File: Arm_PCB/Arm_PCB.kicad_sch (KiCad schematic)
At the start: 28 parts, among them J1 Conn_02x04_Counter_Clockwise, J10 Conn_02x02_Counter_Clockwise, J11 Conn_02x04_Counter_Clockwise, J12 Screw_Terminal_01x02, J13 Screw_Terminal_01x02, J14 Screw_Terminal_01x02, J15 Screw_Terminal_01x02, J16 Screw_Terminal_01x02, J17 Screw_Terminal_01x02, J18 Screw_Terminal_01x02, J2 Conn_02x04_Counter_Clockwise, J3 Conn_02x04_Counter_Clockwise, J4 Conn_02x04_Counter_Clockwise, J5 Conn_02x03_Counter_Clockwise, J7 Conn_02x03_Counter_Clockwise, J8 Conn_02x02_Counter_Clockwise, J9 Conn_02x04_Counter_Clockwise, SW1 SW_Push, SW2 SW_Push, SW3 SW_Push, SW4 SW_Push

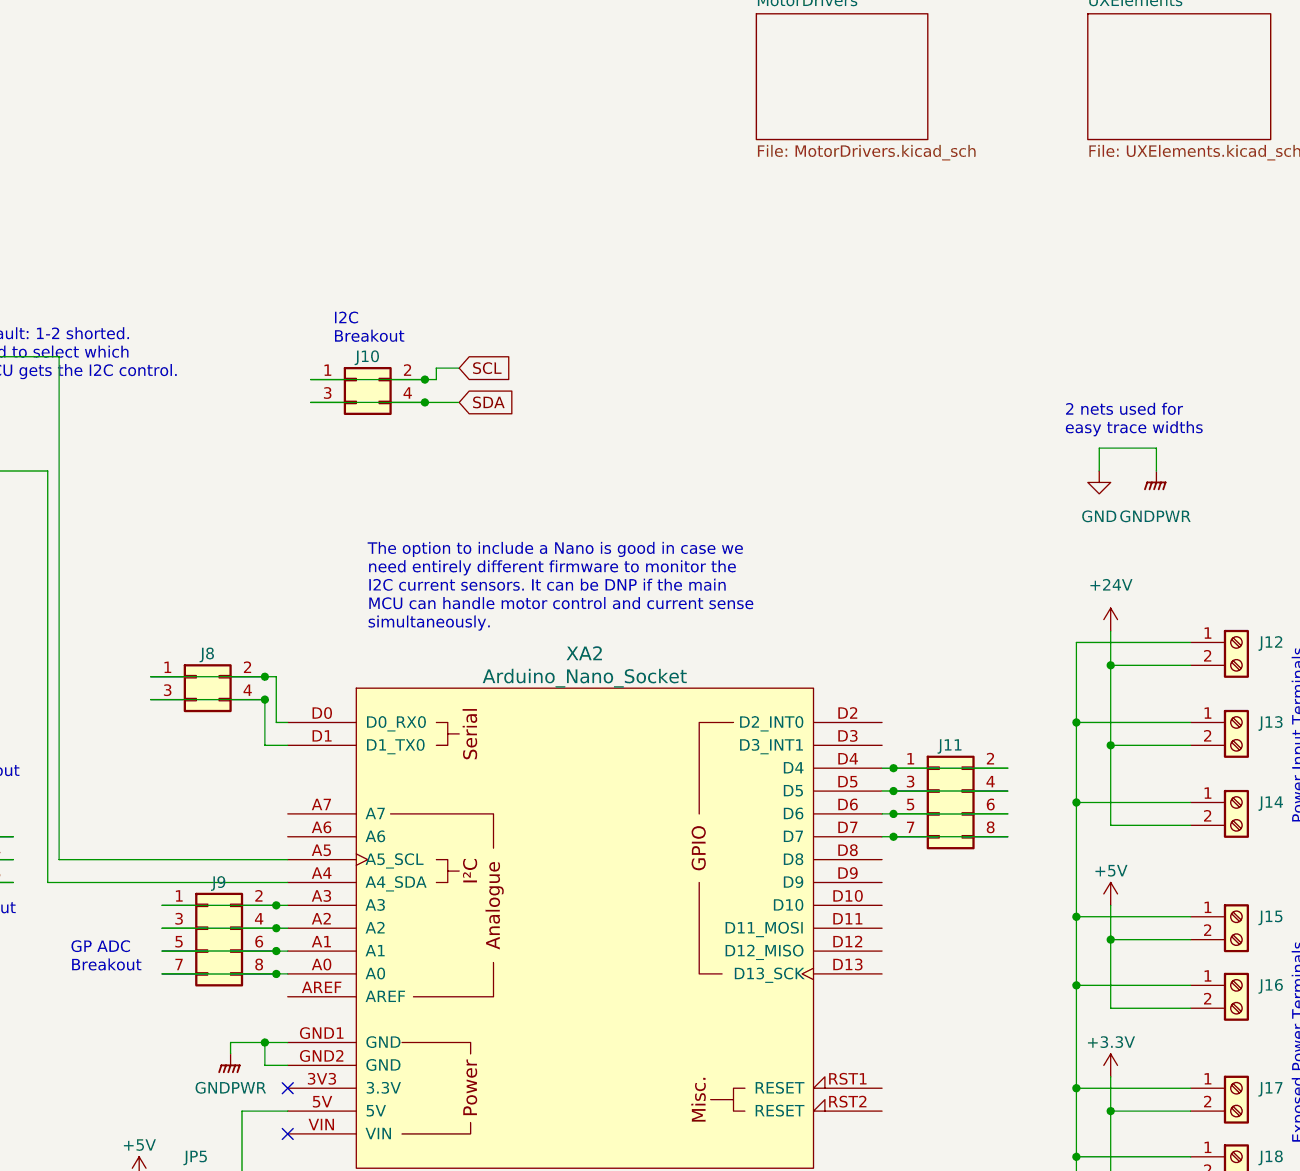
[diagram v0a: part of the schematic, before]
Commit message: Continue layout, pick some components
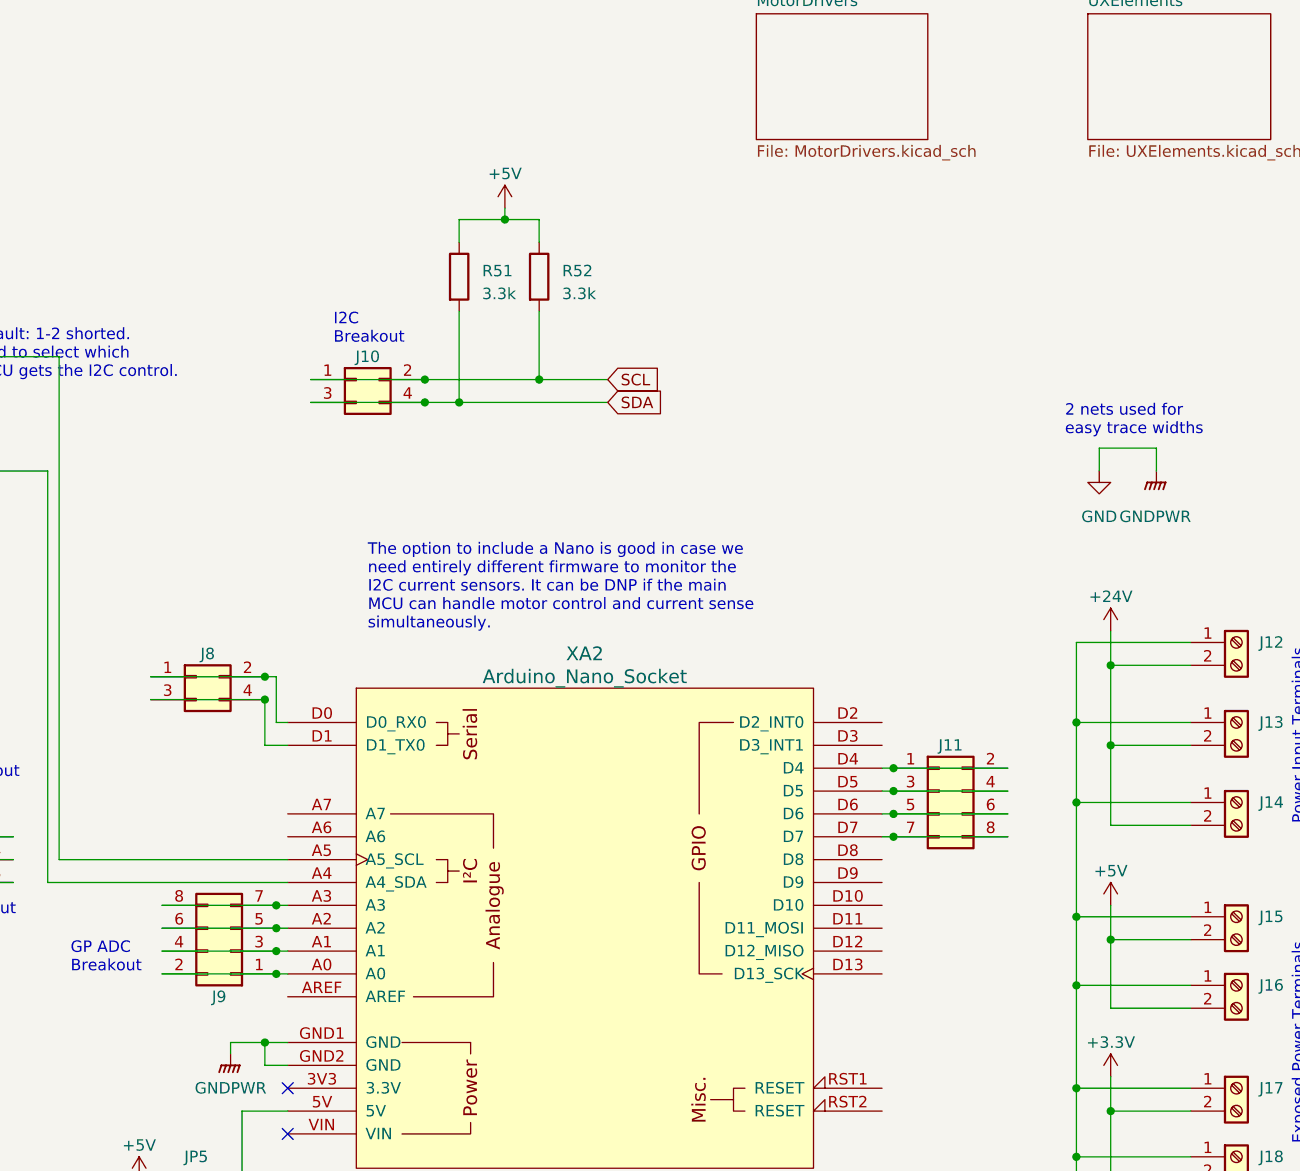
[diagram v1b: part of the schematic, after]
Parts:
- added R51, R52: 3.3k, Resistor_SMD:R_1206_3216Metric_Pad1.30x1.75mm_HandSolder, symbol Device:R
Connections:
- net +5V: now also R51.1, R52.1
- net SCL: now also R52.2
- net SDA: now also R51.2
- net at J9.7 (Pin_7), J9.8 (Pin_8): now also XA2.A3; no longer XA2.A0
- net at J9.5 (Pin_5), J9.6 (Pin_6): now also XA2.A2; no longer XA2.A1
- net at J9.3 (Pin_3), J9.4 (Pin_4): now also XA2.A1; no longer XA2.A2
- net at J9.1 (Pin_1), J9.2 (Pin_2): now also XA2.A0; no longer XA2.A3
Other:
- moved on the sheet: J9
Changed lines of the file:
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@@
   (junction (at 95.25 110.49) (diameter 0) (color 0 0 0 0)
   )
+  (junction (at 176.53 62.23) (diameter 0) (color 0 0 0 0)
+  )
   (junction (at 105.41 118.11) (diameter 0) (color 0 0 0 0)
   )
@@
   (junction (at 24.13 173.99) (diameter 0) (color 0 0 0 0)
   )
+  (junction (at 172.72 44.45) (diameter 0) (color 0 0 0 0)
+  )
   (junction (at 24.13 176.53) (diameter 0) (color 0 0 0 0)
   )
@@
   )
   (junction (at 215.9 113.03) (diameter 0) (color 0 0 0 0)
+  )
+  (junction (at 167.64 64.77) (diameter 0) (color 0 0 0 0)
   )
   (junction (at 26.67 118.11) (diameter 0) (color 0 0 0 0)
@@
   (no_connect (at 148.59 140.97))
   (no_connect (at 27.94 191.77))
+  (wire (pts (xy 176.53 46.99) (xy 176.53 44.45))
+    (stroke (width 0) (type default))
+  )
   (wire (pts (xy 93.98 120.65) (xy 96.52 120.65))
     (stroke (width 0) (type default))
@@
     (stroke (width 0) (type default))
   )
+  (wire (pts (xy 167.64 44.45) (xy 167.64 46.99))
+    (stroke (width 0) (type default))
+  )
   (wire (pts (xy 146.05 97.79) (xy 133.35 97.79))
     (stroke (width 0) (type default))
@@
     (stroke (width 0) (type default))
   )
+  (wire (pts (xy 176.53 54.61) (xy 176.53 62.23))
+    (stroke (width 0) (type default))
+  )
   (wire (pts (xy 95.25 107.95) (xy 107.95 107.95))
     (stroke (width 0) (type default))
@@
     (stroke (width 0) (type default))
   )
+  (wire (pts (xy 172.72 43.18) (xy 172.72 44.45))
+    (stroke (width 0) (type default))
+  )
   (wire (pts (xy 240.03 120.65) (xy 240.03 124.46))
     (stroke (width 0) (type default))
   )
+  (wire (pts (xy 167.64 64.77) (xy 184.15 64.77))
+    (stroke (width 0) (type default))
+  )
   (wire (pts (xy 96.52 125.73) (xy 93.98 125.73))
     (stroke (width 0) (type default))
@@
     (stroke (width 0) (type default))
   )
+  (wire (pts (xy 167.64 54.61) (xy 167.64 64.77))
+    (stroke (width 0) (type default))
+  )
   (wire (pts (xy 240.03 93.98) (xy 248.92 93.98))
     (stroke (width 0) (type default))
@@
     (stroke (width 0) (type default))
   )
+  (wire (pts (xy 172.72 44.45) (xy 167.64 44.45))
+    (stroke (width 0) (type default))
+  )
   (wire (pts (xy 46.99 26.67) (xy 48.26 26.67))
     (stroke (width 0) (type default))
@@
     (stroke (width 0) (type default))
   )
-  (wire (pts (xy 163.83 62.23) (xy 165.1 62.23))
+  (wire (pts (xy 163.83 62.23) (xy 176.53 62.23))
     (stroke (width 0) (type default))
   )
@@
     (stroke (width 0) (type default))
   )
-  (wire (pts (xy 165.1 60.96) (xy 165.1 62.23))
-    (stroke (width 0) (type default))
-  )
   (wire (pts (xy 93.98 179.07) (xy 96.52 179.07))
     (stroke (width 0) (type default))
@@
     (stroke (width 0) (type default))
   )
+  (wire (pts (xy 176.53 62.23) (xy 184.15 62.23))
+    (stroke (width 0) (type default))
+  )
   (wire (pts (xy 24.13 184.15) (xy 24.13 186.69))
     (stroke (width 0) (type default))
@@
     (stroke (width 0) (type default))
   )
+  (wire (pts (xy 176.53 44.45) (xy 172.72 44.45))
+    (stroke (width 0) (type default))
+  )
   (wire (pts (xy 93.98 158.75) (xy 96.52 158.75))
     (stroke (width 0) (type default))
@@
   )
   (wire (pts (xy 44.45 26.67) (xy 44.45 24.13))
-    (stroke (width 0) (type default))
-  )
-  (wire (pts (xy 167.64 60.96) (xy 165.1 60.96))
     (stroke (width 0) (type default))
   )
@@
     )
   )
-  (global_label "SCL" (shape input) (at 167.64 60.96 0) (fields_autoplaced)
-    (effects (font (size 1.27 1.27)) (justify left))
-    (property "Intersheetrefs" "${INTERSHEET_REFS}" (at 173.5607 60.8806 0)
+  (global_label "SCL" (shape input) (at 184.15 62.23 0) (fields_autoplaced)
+    (effects (font (size 1.27 1.27)) (justify left))
+    (property "Intersheetrefs" "${INTERSHEET_REFS}" (at 190.0707 62.1506 0)
       (effects (font (size 1.27 1.27)) (justify left) hide)
     )
@@
     )
   )
-  (global_label "SDA" (shape input) (at 167.64 64.77 0) (fields_autoplaced)
-    (effects (font (size 1.27 1.27)) (justify left))
-    (property "Intersheetrefs" "${INTERSHEET_REFS}" (at 173.6212 64.6906 0)
+  (global_label "SDA" (shape input) (at 184.15 64.77 0) (fields_autoplaced)
+    (effects (font (size 1.27 1.27)) (justify left))
+    (property "Intersheetrefs" "${INTERSHEET_REFS}" (at 190.1312 64.6906 0)
       (effects (font (size 1.27 1.27)) (justify left) hide)
     )
@@
         (path "/f8b9fbb1-757f-4aa8-8e30-7f83a30c7c5f"
           (reference "#PWR09") (unit 1)
+        )
+      )
+    )
+  )
+  (symbol (lib_id "Device:R") (at 176.53 50.8 0) (unit 1)
+    (in_bom yes) (on_board yes) (dnp no) (fields_autoplaced)
+    (property "Reference" "R52" (at 179.07 50.165 0)
+      (effects (font (size 1.27 1.27)) (justify left))
+    )
+    (property "Value" "3.3k" (at 179.07 52.705 0)
+      (effects (font (size 1.27 1.27)) (justify left))
+    )
+    (property "Footprint" "Resistor_SMD:R_1206_3216Metric_Pad1.30x1.75mm_HandSolder" (at 174.752 50.8 90)
+      (effects (font (size 1.27 1.27)) hide)
+    )
+    (property "Datasheet" "~" (at 176.53 50.8 0)
+      (effects (font (size 1.27 1.27)) hide)
+    )
+    (pin "1")
+    (pin "2")
+    (instances
+      (project "Arm_PCB"
+        (path "/f8b9fbb1-757f-4aa8-8e30-7f83a30c7c5f"
+          (reference "R52") (unit 1)
         )
       )
@@
     )
   )
+  (symbol (lib_name "+5V_1") (lib_id "power:+5V") (at 172.72 43.18 0) (unit 1)
+    (in_bom yes) (on_board yes) (dnp no)
+    (property "Reference" "#PWR080" (at 172.72 46.99 0)
+      (effects (font (size 1.27 1.27)) hide)
+    )
+    (property "Value" "+5V" (at 172.72 39.37 0)
+      (effects (font (size 1.27 1.27)))
+    )
+    (property "Footprint" "" (at 172.72 43.18 0)
+      (effects (font (size 1.27 1.27)) hide)
+    )
+    (property "Datasheet" "" (at 172.72 43.18 0)
+      (effects (font (size 1.27 1.27)) hide)
+    )
+    (pin "1")
+    (instances
+      (project "Arm_PCB"
+        (path "/f8b9fbb1-757f-4aa8-8e30-7f83a30c7c5f"
+          (reference "#PWR080") (unit 1)
+        )
+      )
+    )
+  )
   (symbol (lib_id "Connector:Screw_Terminal_01x02") (at 254 100.33 0) (unit 1)
     (in_bom yes) (on_board yes) (dnp no) (fields_autoplaced)
@@
     )
   )
+  (symbol (lib_id "Device:R") (at 167.64 50.8 0) (unit 1)
+    (in_bom yes) (on_board yes) (dnp no) (fields_autoplaced)
+    (property "Reference" "R51" (at 170.18 50.165 0)
+      (effects (font (size 1.27 1.27)) (justify left))
+    )
+    (property "Value" "3.3k" (at 170.18 52.705 0)
+      (effects (font (size 1.27 1.27)) (justify left))
+    )
+    (property "Footprint" "Resistor_SMD:R_1206_3216Metric_Pad1.30x1.75mm_HandSolder" (at 165.862 50.8 90)
+      (effects (font (size 1.27 1.27)) hide)
+    )
+    (property "Datasheet" "~" (at 167.64 50.8 0)
+      (effects (font (size 1.27 1.27)) hide)
+    )
+    (pin "1")
+    (pin "2")
+    (instances
+      (project "Arm_PCB"
+        (path "/f8b9fbb1-757f-4aa8-8e30-7f83a30c7c5f"
+          (reference "R51") (unit 1)
+        )
+      )
+    )
+  )
   (symbol (lib_id "Connector_Generic:Conn_02x02_Odd_Even") (at 156.21 62.23 0) (unit 1)
     (in_bom yes) (on_board yes) (dnp no)
@@
   )
   (symbol (lib_id "power:+24V") (at 240.03 90.17 0) (unit 1)
-    (in_bom yes) (on_board yes) (dnp no) (fields_autoplaced)
+    (in_bom yes) (on_board yes) (dnp no)
     (property "Reference" "#PWR014" (at 240.03 93.98 0)
       (effects (font (size 1.27 1.27)) hide)
     )
-    (property "Value" "+24V" (at 240.03 85.09 0)
+    (property "Value" "+24V" (at 240.03 86.36 0)
       (effects (font (size 1.27 1.27)))
     )
@@
     )
   )
-  (symbol (lib_id "Connector_Generic:Conn_02x04_Odd_Even") (at 139.7 123.19 0) (unit 1)
-    (in_bom yes) (on_board yes) (dnp no)
-    (property "Reference" "J9" (at 140.97 118.11 0)
-      (effects (font (size 1.27 1.27)))
-    )
-    (property "Value" "Conn_02x04_Counter_Clockwise" (at 140.97 118.11 0)
-      (effects (font (size 1.27 1.27)) hide)
-    )
-    (property "Footprint" "Connector_PinHeader_2.54mm:PinHeader_2x04_P2.54mm_Vertical" (at 139.7 123.19 0)
-      (effects (font (size 1.27 1.27)) hide)
-    )
-    (property "Datasheet" "~" (at 139.7 123.19 0)
-      (effects (font (size 1.27 1.27)) hide)
-    )
+  (symbol (lib_id "Connector_Generic:Conn_02x04_Odd_Even") (at 142.24 125.73 180) (unit 1)
+    (in_bom yes) (on_board yes) (dnp no)
+    (property "Reference" "J9" (at 140.97 130.81 0)
+      (effects (font (size 1.27 1.27)))
+    )
+    (property "Value" "Conn_02x04_Counter_Clockwise" (at 140.97 130.81 0)
+      (effects (font (size 1.27 1.27)) hide)
+    )
+    (property "Footprint" "Connector_PinHeader_2.54mm:PinHeader_2x04_P2.54mm_Vertical" (at 142.24 125.73 0)
+      (effects (font (size 1.27 1.27)) hide)
+    )
+    (property "Datasheet" "~" (at 142.24 125.73 0)
+      (effects (font (size 1.27 1.27)) hide)
+    )
